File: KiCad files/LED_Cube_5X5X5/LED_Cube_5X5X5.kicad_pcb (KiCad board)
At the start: 2 copper layers, 100 x 100 mm, 66 parts, among them J1 Barrel_Jack_MountingPin, J2 USBASP, J3 CON1, J4 CON2, J5 CON3, Q1 BC337, Q2 BC337, Q3 BC337, Q4 BC337, Q5 BC337, SW1 RESET, U1 ATmega16-16PU, U2 74HC595, U3 74HC595, U4 74HC595, U5 74HC595, Y1 16MHz

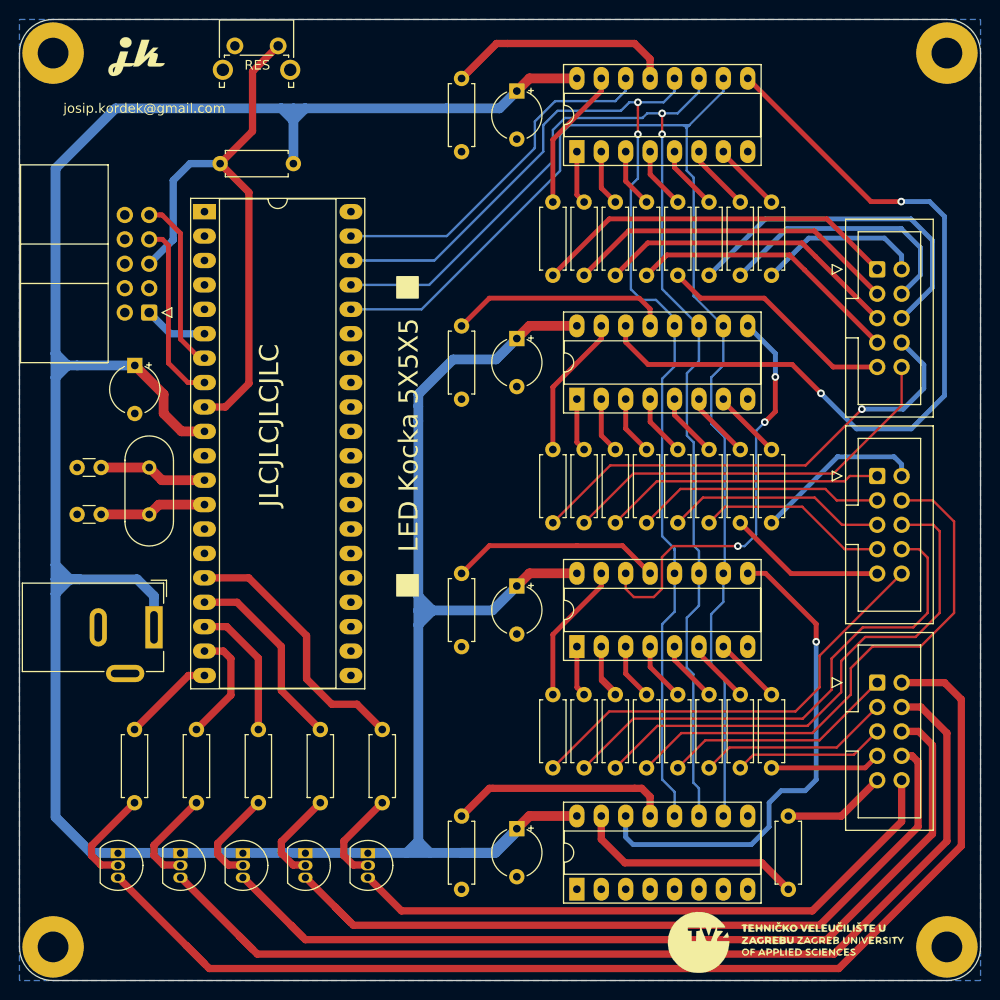
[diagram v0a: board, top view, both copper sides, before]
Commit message: 3d model
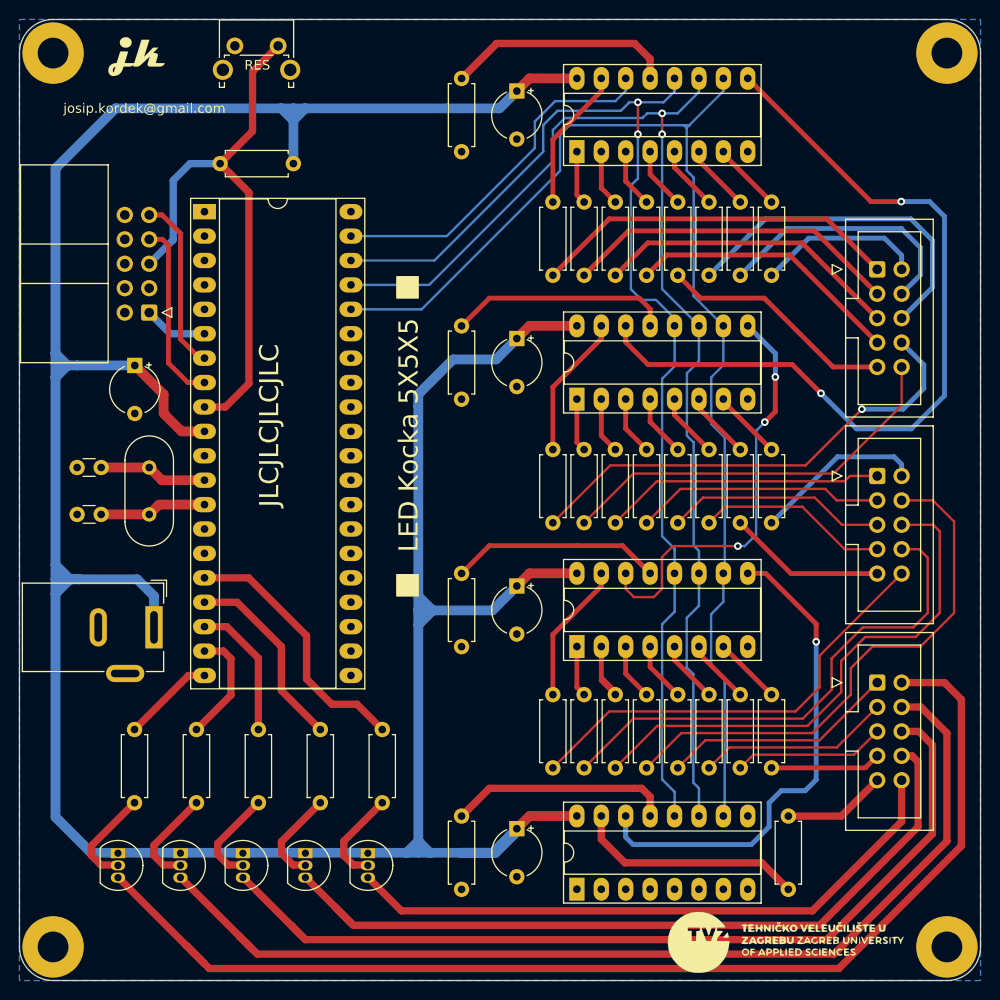
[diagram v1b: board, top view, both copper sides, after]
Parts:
- J1: footprint Connector_BarrelJack:BarrelJack_Wuerth_6941xx301002 -> Footprints:BarrelJack_Wuerth_6941xx301002
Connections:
- J2 pad 2: Net-(J2-Pad2) -> unconnected-(J2-Pad2)
- J2 pad 3: Net-(J2-Pad3) -> unconnected-(J2-Pad3)
- J2 pad 4: Net-(J2-Pad4) -> unconnected-(J2-Pad4)
- J2 pad 6: Net-(J2-Pad6) -> unconnected-(J2-Pad6)
- J2 pad 8: Net-(J2-Pad8) -> unconnected-(J2-Pad8)
- U1 pad 1: Net-(U1-Pad1) -> unconnected-(U1-Pad1)
- U1 pad 14: Net-(U1-Pad14) -> unconnected-(U1-Pad14)
- U1 pad 15: Net-(U1-Pad15) -> unconnected-(U1-Pad15)
- U1 pad 2: Net-(U1-Pad2) -> unconnected-(U1-Pad2)
- U1 pad 21: Net-(U1-Pad21) -> unconnected-(U1-Pad21)
- U1 pad 22: Net-(U1-Pad22) -> unconnected-(U1-Pad22)
- U1 pad 23: Net-(U1-Pad23) -> unconnected-(U1-Pad23)
- U1 pad 24: Net-(U1-Pad24) -> unconnected-(U1-Pad24)
- U1 pad 25: Net-(U1-Pad25) -> unconnected-(U1-Pad25)
- U1 pad 26: Net-(U1-Pad26) -> unconnected-(U1-Pad26)
- U1 pad 27: Net-(U1-Pad27) -> unconnected-(U1-Pad27)
- U1 pad 28: Net-(U1-Pad28) -> unconnected-(U1-Pad28)
- U1 pad 29: Net-(U1-Pad29) -> unconnected-(U1-Pad29)
- U1 pad 3: Net-(U1-Pad3) -> unconnected-(U1-Pad3)
- U1 pad 30: Net-(U1-Pad30) -> unconnected-(U1-Pad30)
- U1 pad 32: Net-(U1-Pad32) -> unconnected-(U1-Pad32)
- U1 pad 33: Net-(U1-Pad33) -> unconnected-(U1-Pad33)
- U1 pad 34: Net-(U1-Pad34) -> unconnected-(U1-Pad34)
- U1 pad 35: Net-(U1-Pad35) -> unconnected-(U1-Pad35)
- U1 pad 4: Net-(U1-Pad4) -> unconnected-(U1-Pad4)
- U1 pad 40: Net-(U1-Pad40) -> unconnected-(U1-Pad40)
- U1 pad 5: Net-(U1-Pad5) -> unconnected-(U1-Pad5)
- U5 pad 1: Net-(U5-Pad1) -> unconnected-(U5-Pad1)
- U5 pad 2: Net-(U5-Pad2) -> unconnected-(U5-Pad2)
- U5 pad 3: Net-(U5-Pad3) -> unconnected-(U5-Pad3)
- U5 pad 4: Net-(U5-Pad4) -> unconnected-(U5-Pad4)
- U5 pad 5: Net-(U5-Pad5) -> unconnected-(U5-Pad5)
- U5 pad 6: Net-(U5-Pad6) -> unconnected-(U5-Pad6)
- U5 pad 7: Net-(U5-Pad7) -> unconnected-(U5-Pad7)
- U5 pad 9: Net-(U5-Pad9) -> unconnected-(U5-Pad9)
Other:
- net class Default removed
